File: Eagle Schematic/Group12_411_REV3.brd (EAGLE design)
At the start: 58.4 x 45.4 mm, 32 parts, among them J2 5.5x2.1mm Barrel, Q1 600mA/40V, T1 2N7002F, U1 STMICROELECTRONICS_L7805ABD2T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, U2 ATMEGA32U4-AU, X2 ABLS-16.000MHZ-B4-T

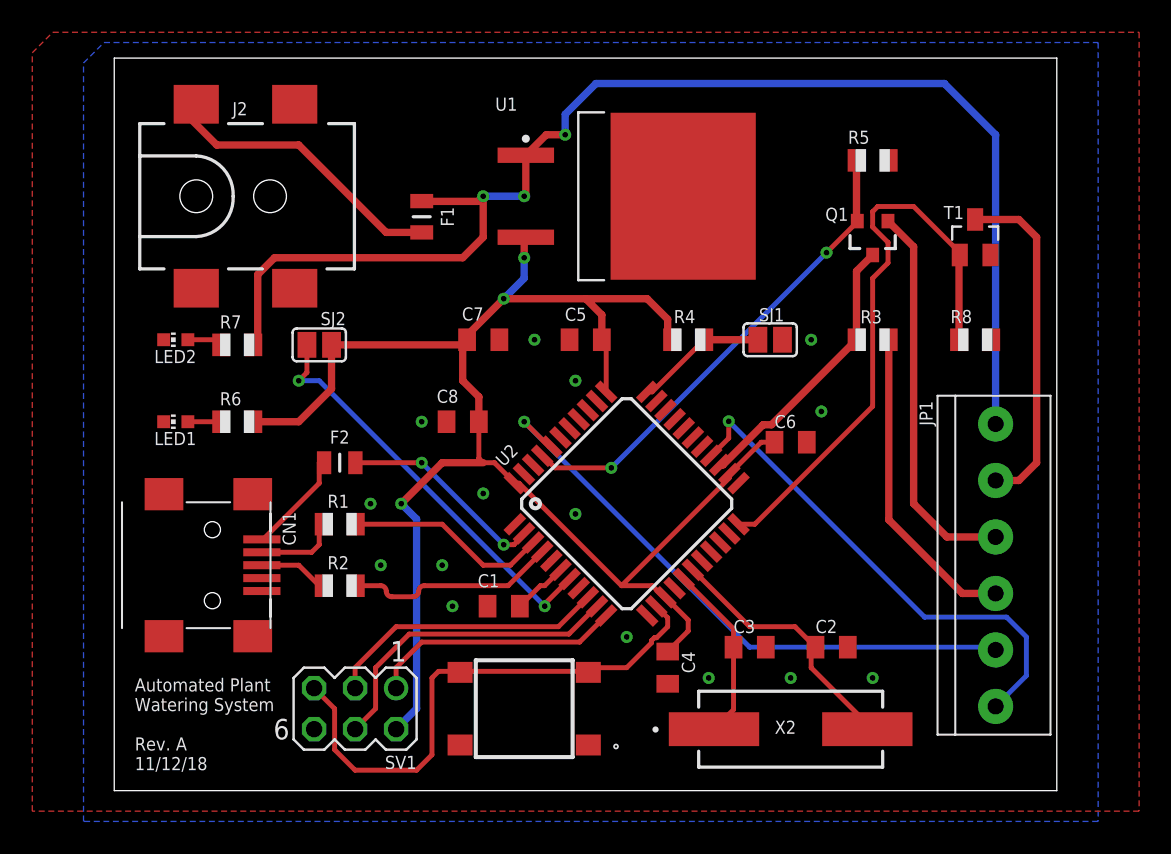
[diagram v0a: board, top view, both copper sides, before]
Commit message: Cross your fingers
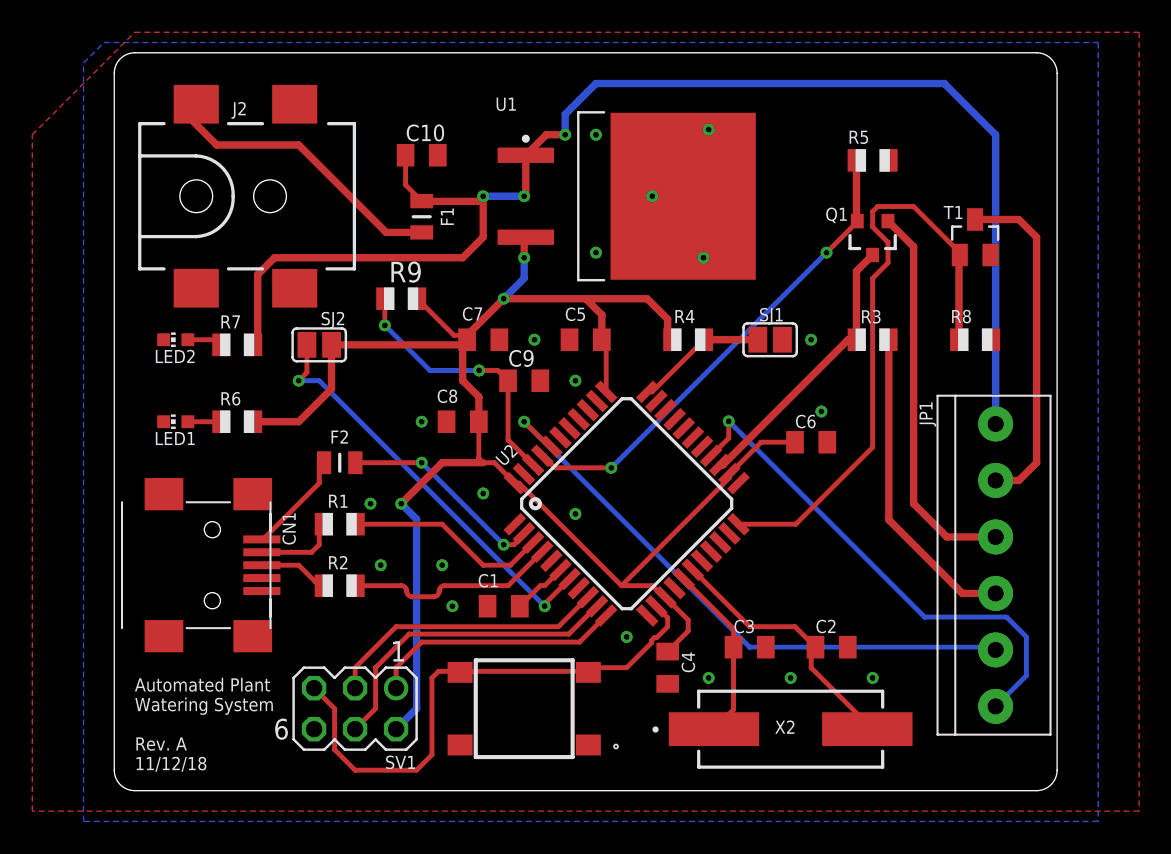
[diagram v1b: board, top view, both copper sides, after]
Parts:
- added C10: 10uF, adafruit:C0805K
- added C9: 0.1uF, adafruit:C0805K
- added R9: 100k, adafruit:R0805
- moved C6 1.27 mm to (50.8, 31.8)
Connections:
- new net N$23: C9.1, R9.1, U2.42
- new net N$25: C9.2
- net 12V: now also C10.1
- net GND: now also C10.2
- net VCC: now also R9.2
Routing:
- net N$23: track 0.00 -> 16.6 mm, vias 0 -> 2
- net VCC: track 105.3 -> 110.6 mm
- net 12V: track 81.6 -> 85.2 mm
- net N$18: track 36.3 -> 37.8 mm
- net GND: vias 15 -> 18
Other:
- board size 58.4 x 45.4 mm -> 58.4 x 45.7 mm
